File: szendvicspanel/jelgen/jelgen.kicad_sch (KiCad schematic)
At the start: 23 parts, among them J1 Conn_01x04_Pin, U1 TL072, U2 TL072

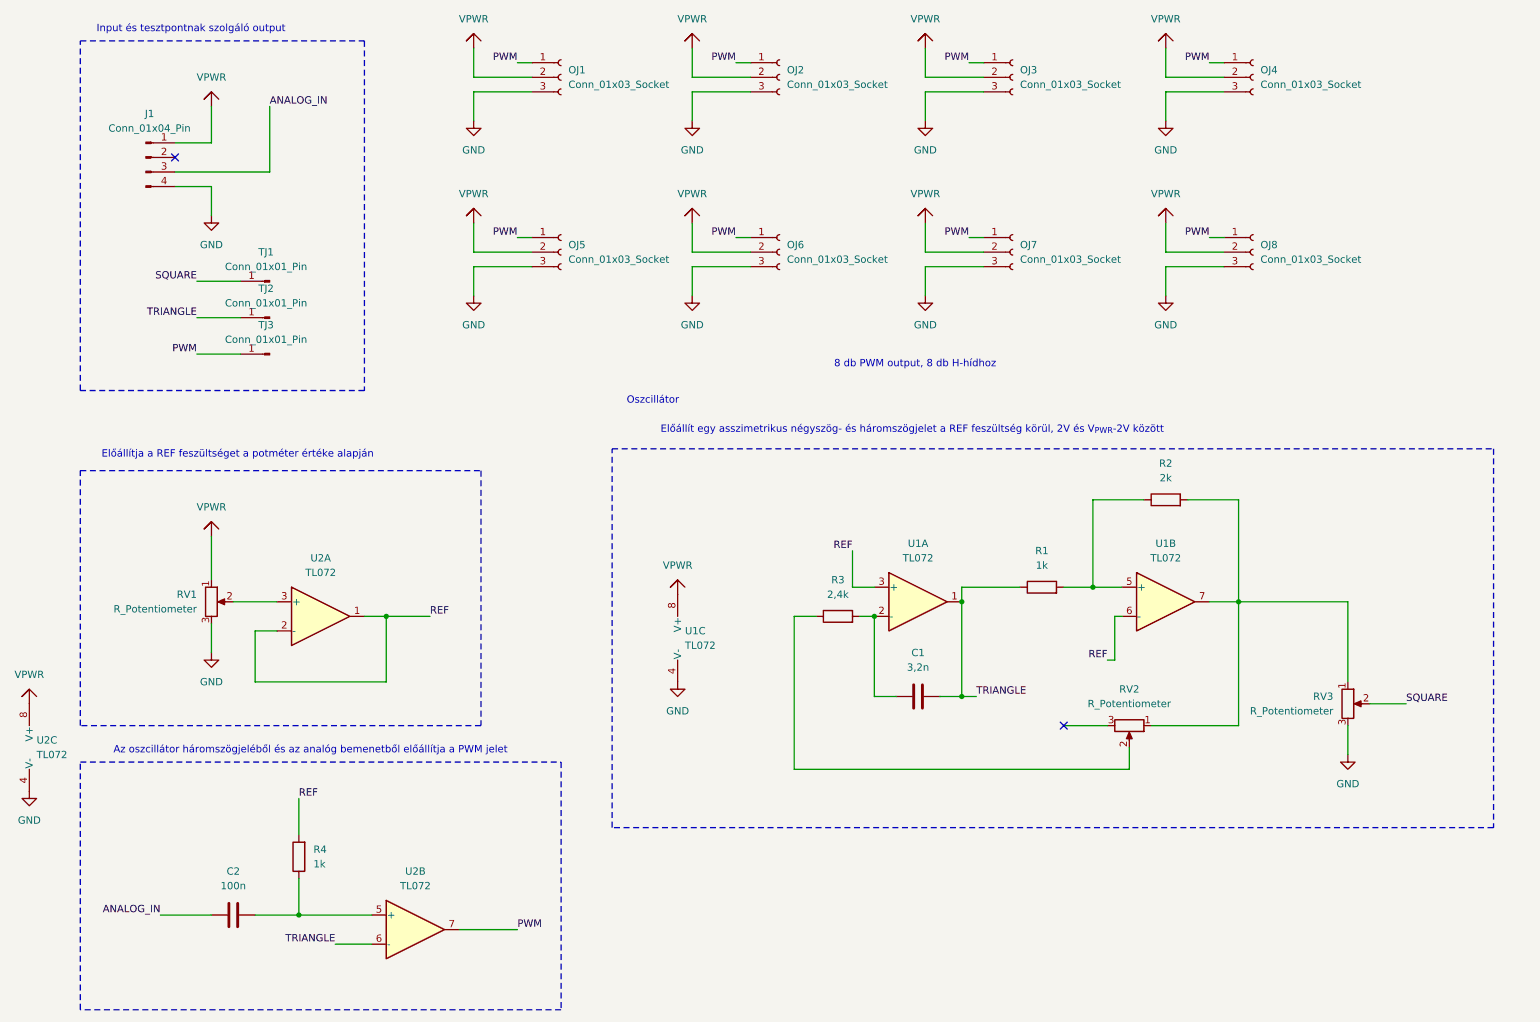
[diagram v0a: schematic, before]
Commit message: PCB sketch 2
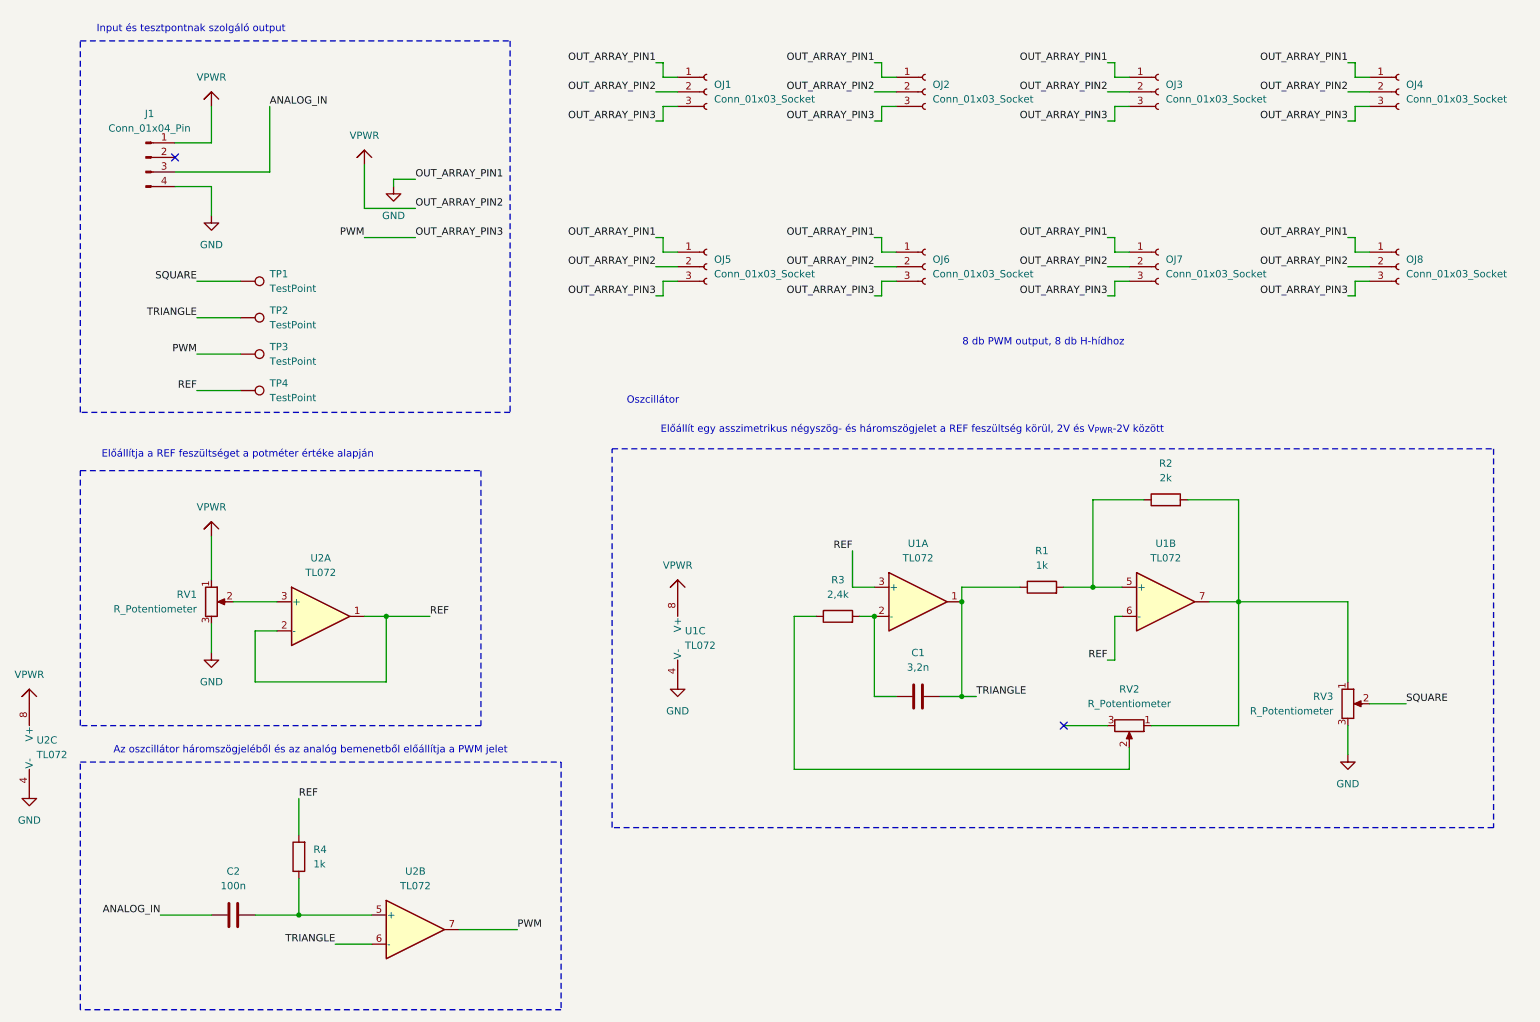
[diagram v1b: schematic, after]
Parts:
- removed TJ1, TJ2, TJ3: Conn_01x01_Pin, Connector_PinHeader_2.54mm:PinHeader_1x01_P2.54mm_Vertical, symbol Connector:Conn_01x01_Pin
- added TP1, TP2, TP3, TP4: TestPoint, Connector_PinHeader_2.54mm:PinHeader_1x01_P2.54mm_Vertical, symbol Connector:TestPoint
- J1: footprint Connector_PinHeader_2.54mm:PinHeader_1x04_P2.54mm_Horizontal -> Connector_PinHeader_2.54mm:PinHeader_1x04_P2.54mm_Vertical
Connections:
- net GND: now also OJ1.1 (Pin_1), OJ2.1 (Pin_1), OJ3.1 (Pin_1), OJ4.1 (Pin_1), OJ5.1 (Pin_1), OJ6.1 (Pin_1), OJ7.1 (Pin_1), OJ8.1 (Pin_1); no longer OJ1.3 (Pin_3), OJ2.3 (Pin_3), OJ3.3 (Pin_3), OJ4.3 (Pin_3), OJ5.3 (Pin_3), OJ6.3 (Pin_3), OJ7.3 (Pin_3), OJ8.3 (Pin_3)
- net REF: now also TP4.1
- net SQUARE: now also TP1.1
- net TRIANGLE: now also TP2.1
- removed net PWM: OJ1.1 (Pin_1), OJ2.1 (Pin_1), OJ3.1 (Pin_1), OJ4.1 (Pin_1), OJ5.1 (Pin_1), OJ6.1 (Pin_1), OJ7.1 (Pin_1), OJ8.1 (Pin_1), U2.7
- new net OUT_ARRAY_PIN3: OJ1.3 (Pin_3), OJ2.3 (Pin_3), OJ3.3 (Pin_3), OJ4.3 (Pin_3), OJ5.3 (Pin_3), OJ6.3 (Pin_3), OJ7.3 (Pin_3), OJ8.3 (Pin_3), TP3.1, U2.7
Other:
- moved on the sheet: OJ1, OJ2, OJ3, OJ4, OJ5, OJ6, OJ7, OJ8
